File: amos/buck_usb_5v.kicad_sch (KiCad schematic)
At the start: 15 parts, among them U501 TPS54560DDAR

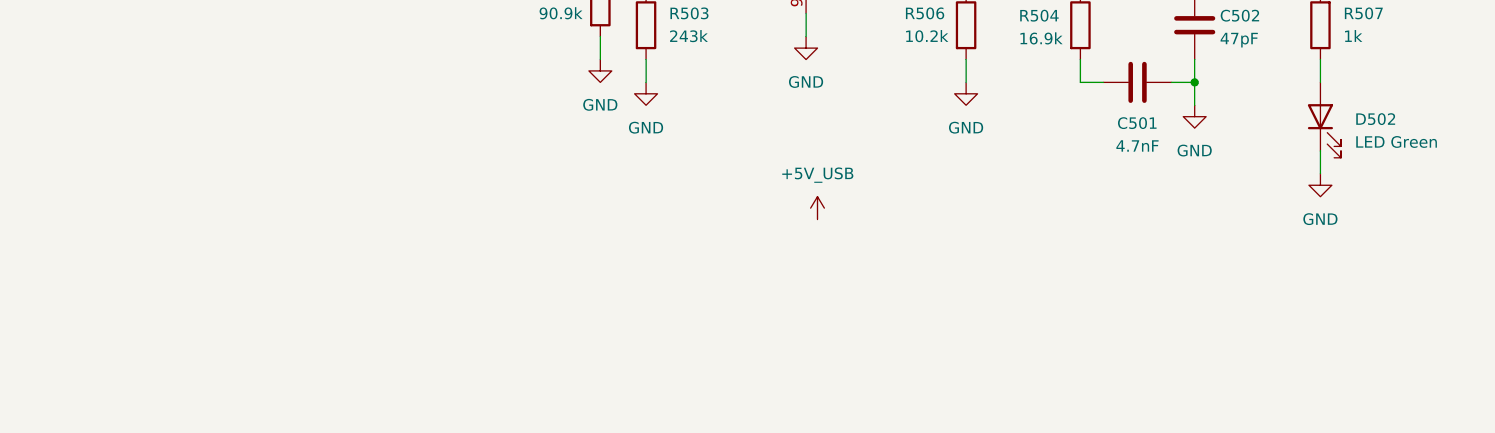
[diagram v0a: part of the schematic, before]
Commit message: update
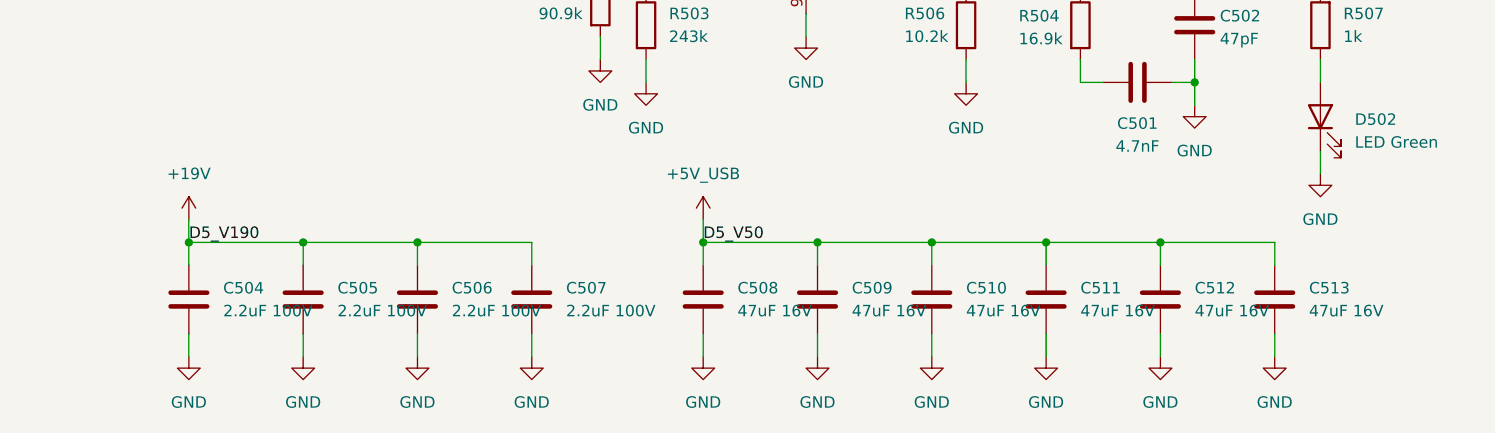
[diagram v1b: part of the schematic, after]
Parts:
- added C504, C505, C506, C507: 2.2uF 100V, Capacitor_SMD:C_1210_3225Metric, symbol Device:C
- added C508, C509, C510, C511, C512, C513: 47uF 16V, Capacitor_SMD:C_1210_3225Metric, symbol Device:C
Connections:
- net +19V: now also C504.1, C505.1, C506.1, C507.1
- net +5V_USB: now also C508.1, C509.1, C510.1, C511.1, C512.1, C513.1
- net GND: now also C504.2, C505.2, C506.2, C507.2, C508.2, C509.2, C510.2, C511.2, C512.2, C513.2
